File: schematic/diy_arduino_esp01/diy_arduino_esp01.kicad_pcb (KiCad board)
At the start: 2 copper layers, 63 x 77 mm, 27 parts, among them J1 ESP 01S SOCKET, J10 3.3v+gnd, J2 programmer, J3 Barrel_Jack, J4 D5-D8, J5 RFID, J6 magnetic reed, J7 A0-A5, J8 RFID, J9 5v+gnd, SW1 SW_Push, U1 ATmega328-P, U2 LM7805_TO220, U4 LM1117T-3.3, Y1 Crystal

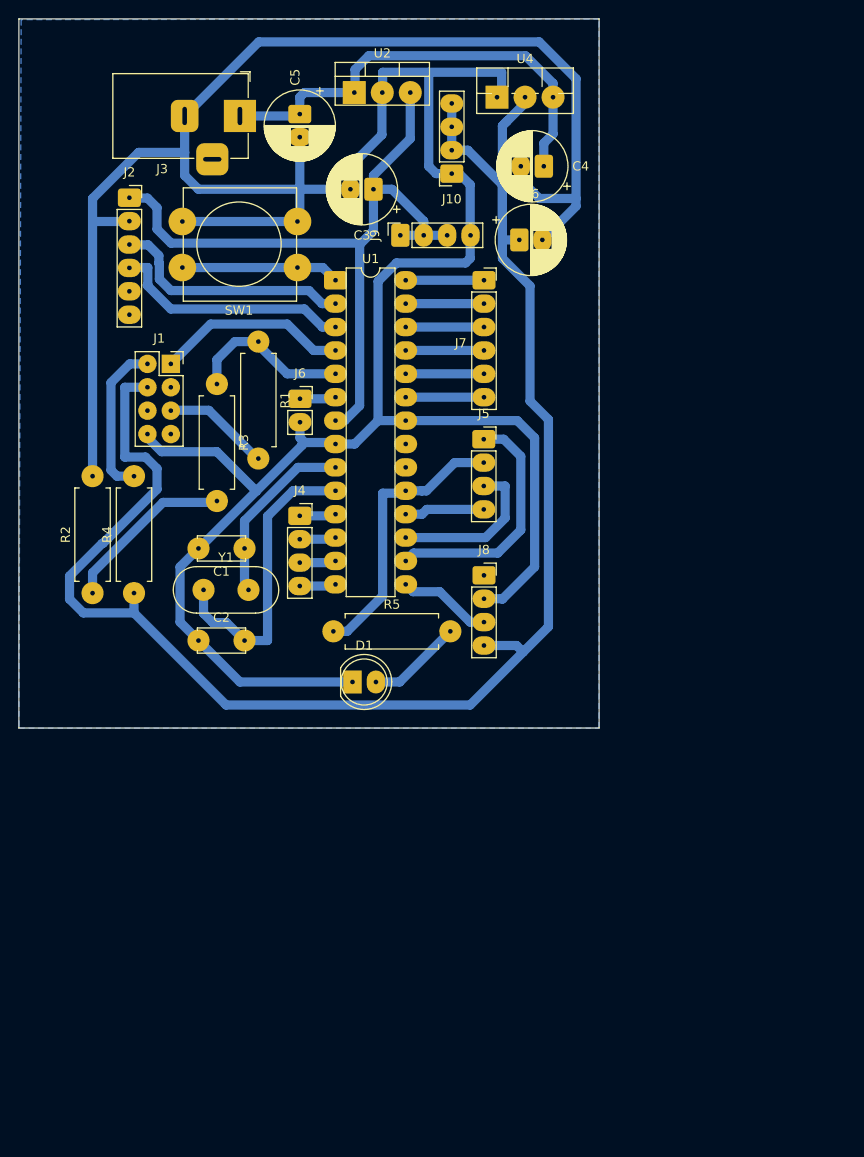
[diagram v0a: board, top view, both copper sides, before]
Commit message: updated schematic
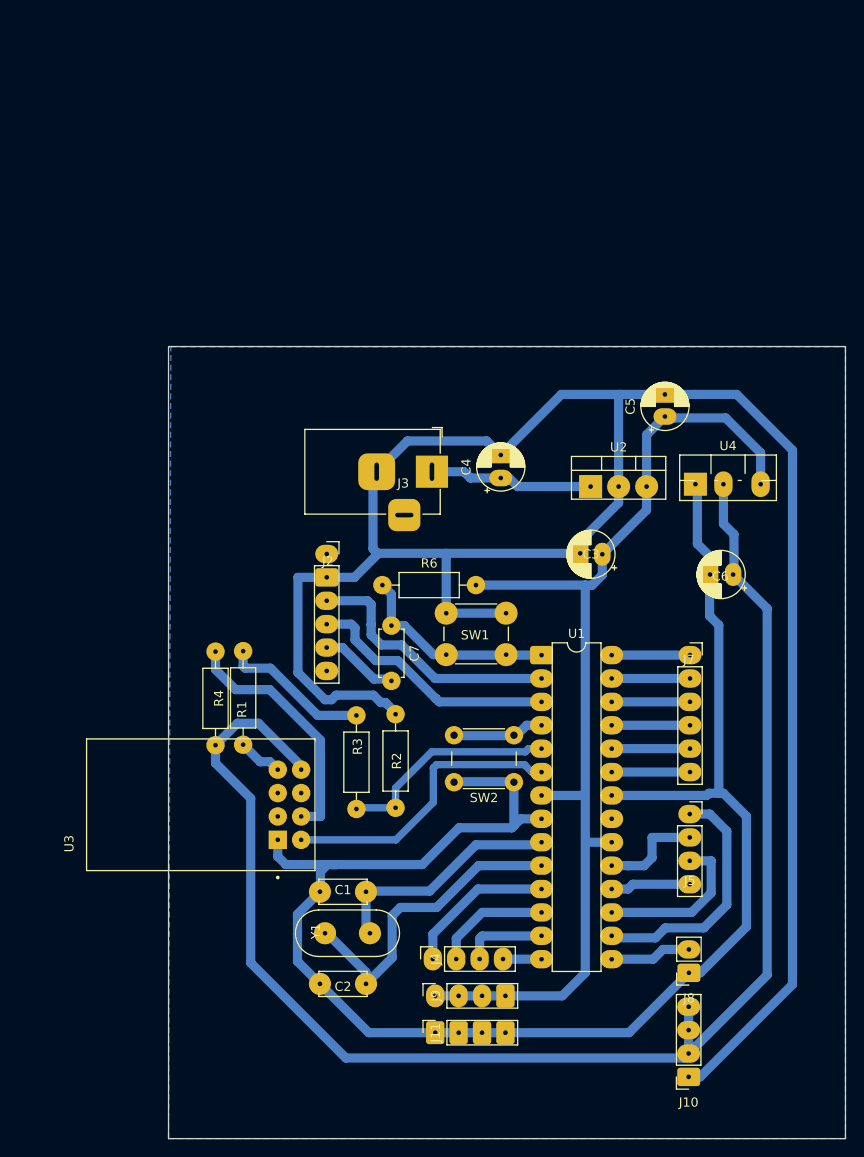
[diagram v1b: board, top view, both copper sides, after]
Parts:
- removed D1: LED, LED_THT:LED_D5.0mm
- removed J1: ESP 01S SOCKET, Connector_PinSocket_2.54mm:PinSocket_2x04_P2.54mm_Vertical
- removed J6: magnetic reed, Connector_PinSocket_2.54mm:PinSocket_1x02_P2.54mm_Vertical
- removed R5: 500, Resistor_THT:R_Axial_DIN0411_L9.9mm_D3.6mm_P12.70mm_Horizontal
- added C7: 0.1uF, Capacitor_THT:C_Disc_D5.0mm_W2.5mm_P5.00mm, F.Cu at (147.2, 86.8)
- added J11: gnd, Connector_PinSocket_2.54mm:PinSocket_1x04_P2.54mm_Vertical, F.Cu at (152.0, 130.5)
- added R6: 500, Resistor_THT:R_Axial_DIN0207_L6.3mm_D2.5mm_P10.16mm_Horizontal, F.Cu at (146.2, 81.9)
- added SW2: hardware interupt, Button_Switch_THT:SW_PUSH_6mm, F.Cu at (160.5, 103.0)
- added U3: ESP-01, ESP-01:MODULE_ESP-01, F.Cu at (126.5, 105.8)
- C3, C4: footprint Capacitor_THT:CP_Radial_D7.5mm_P2.50mm -> Capacitor_THT:CP_Radial_D5.0mm_P2.00mm
- C5, C6: value 16V 1uF -> 16V 10uF; footprint Capacitor_THT:CP_Radial_D7.5mm_P2.50mm -> Capacitor_THT:CP_Radial_D5.0mm_P2.00mm
- J10: value 3.3v+gnd -> 3.3v
- J2: value programmer -> CP0102
- J4: value D5-D8 -> D5
- J7: value A0-A5 -> Anaolg Pins
- J8: footprint Connector_PinSocket_2.54mm:PinSocket_1x04_P2.54mm_Vertical -> Connector_PinSocket_2.54mm:PinSocket_1x02_P2.54mm_Vertical
- J9: value 5v+gnd -> 5V
- R1, R2, R3, R4: footprint Resistor_THT:R_Axial_DIN0411_L9.9mm_D3.6mm_P12.70mm_Horizontal -> Resistor_THT:R_Axial_DIN0207_L6.3mm_D2.5mm_P10.16mm_Horizontal
- SW1: footprint Button_Switch_THT:SW_PUSH-12mm_Wuerth-430476085716 -> Button_Switch_THT:SW_PUSH_6mm
- Y1: footprint Crystal:Crystal_HC49-4H_Vertical -> Crystal:Crystal_HC49-U_Vertical
- moved J10 101.4 mm to (179.5, 135.3)
- moved J9 82.7 mm to (152.0, 126.5)
- moved C5 51.4 mm to (176.9, 63.5), turned to 90 degrees
- moved J4 50.2 mm to (151.7, 122.5), turned to 90 degrees
- moved U2 49.9 mm to (169.3, 71.2)
- moved J8 48.6 mm to (179.5, 124.0), turned to 180 degrees
- moved SW1 47.7 mm to (159.7, 89.5)
- moved U4 47.5 mm to (181.2, 70.9)
- moved C3 46.7 mm to (169.9, 78.5)
- moved J5 46.4 mm to (179.6, 106.8)
- moved J7 46.4 mm to (179.6, 89.5)
- moved U1 46.4 mm to (163.5, 89.5)
- moved J2 44.2 mm to (140.2, 78.5)
- moved J3 43.9 mm to (151.6, 69.6)
- moved C6 43.0 mm to (184.0, 80.8), turned to 180 degrees
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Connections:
- net D5 renamed D5/REED
- net D6 renamed D6/servo
- net D7 renamed D7/relay
- net D8 renamed D8/PIR
- net MISO renamed D12/MISO
- net MOSI renamed D11/MOSI
- net Net-(J2-Pin_3) renamed RX
- net Net-(J2-Pin_4) renamed TX
- net SCK renamed D13/SCK
- net SDA renamed D10/SDA
- C4 pad 1: Net-(U2-VI) -> VCC
- C5 pad 1: Net-(U2-VI) -> 5V
- J2 pad 1: 5V -> unconnected-(J2-Pin_1-Pad1)
- J2 pad 5: unconnected-(J2-Pin_5-Pad5) -> Net-(J2-Pin_5)
- J3 pad 1: Net-(U2-VI) -> VCC
- J8 pad 1: unconnected-(J8-Pin_1-Pad1) -> GND
- J8 pad 2: GND -> D9/RST
- J9 pad 4: GND -> 5V
- R1 pad 1: Net-(U1-PD3) -> Net-(R1-Pad1)
- R2 pad 1: Net-(R2-Pad1) -> D3
- R3 pad 1: Net-(U1-PD3) -> Net-(R1-Pad1)
- R3 pad 2: Net-(R2-Pad1) -> D3
- R4 pad 1: 3.3V -> Net-(U3-CH_PD)
- R4 pad 2: Net-(J1-Pin_2) -> 3.3V
- U1 pad 15: RST -> D9/RST
- U1 pad 20: unconnected-(U1-AVCC-Pad20) -> 5V
- U1 pad 4: Net-(J1-Pin_1) -> D2/Interupt
- U1 pad 5: Net-(U1-PD3) -> D3
- U2 pad 1: Net-(U2-VI) -> VCC
- U4 pad 3: Net-(U2-VI) -> 5V
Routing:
- net Net-(U2-VI): track 49.9 -> 0.00 mm
- net GND: track 358.8 -> 399.1 mm
- net 5V: track 81.2 -> 116.1 mm
- net D4: track 3.93 -> 32.4 mm
- net Net-(U3-CH_PD): track 0.00 -> 26.9 mm
- net D3: track 0.00 -> 24.1 mm
- net Net-(J1-Pin_1): track 20.9 -> 0.00 mm
- net D13/SCK: track 30.5 -> 11.4 mm
- net Net-(R2-Pad1): track 18.9 -> 0.00 mm
- net VCC: track 0.00 -> 17.9 mm
- net Net-(U1-PD3): track 17.6 -> 0.00 mm
- net Net-(J1-Pin_2): track 17.1 -> 0.00 mm
- net Net-(R1-Pad1): track 0.00 -> 16.1 mm
- net 3.3V: track 177.8 -> 163.9 mm
- net D5/REED: track 3.95 -> 16.8 mm
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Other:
- board size 63 x 77 mm -> 73.5 x 86 mm
- board text added: "3.3V"
- board text added: "5v"
- board text added: "<- | | | | | | | | <-"
- board text added: "<- | | | | | | | | | | | | <-"
- board text added: "<-5V"
- board text added: "A0"
- board text added: "A1"
- board text added: "A2"
- board text added: "A3"
- board text added: "A4"
- board text added: "A5"
- board text added: "D10/SDA"
- board text added: "D11/MOSI"
- board text added: "D12/MISO"
- board text added: "D13/SCK"
- board text added: "D2"
- board text added: "D6/servo"
- board text added: "D7/RELAY"
- board text added: "D8/PIR"
- board text added: "D9/RST"
- board text added: "EN"
- board text added: "GND"
- board text added: "GND->"
- board text added: "Hardware"
- board text added: "Interrupt"
- board text added: "RX"
- board text added: "TX"
- board text added: "^"
- board text added: "|"
